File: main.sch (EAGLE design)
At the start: 31 parts, among them IC1 ATTINY13A-SSH, T1A 2N4401, T1B NPN, T2A 2N4401, T2B NPN

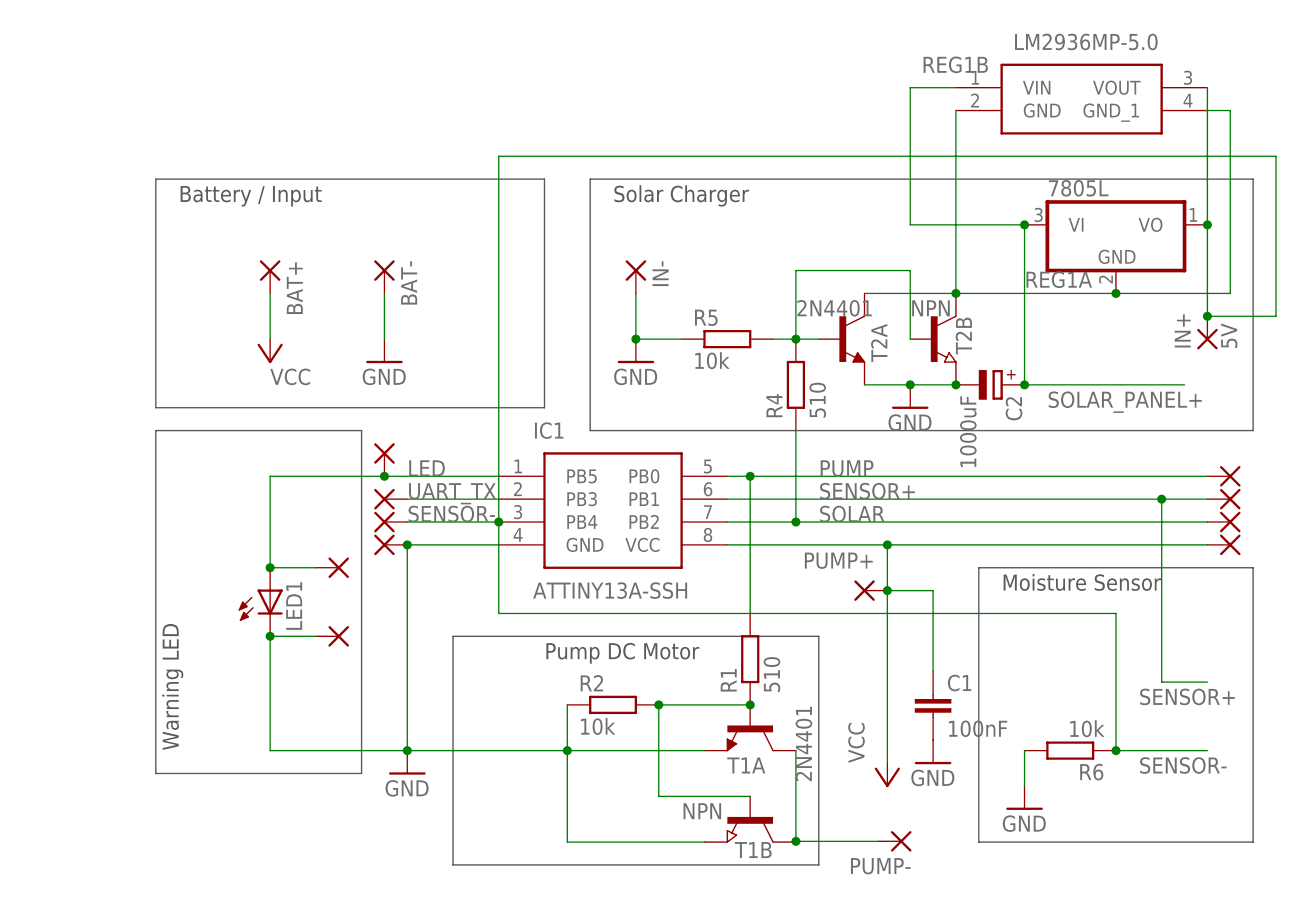
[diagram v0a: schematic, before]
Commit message: rev 0.6
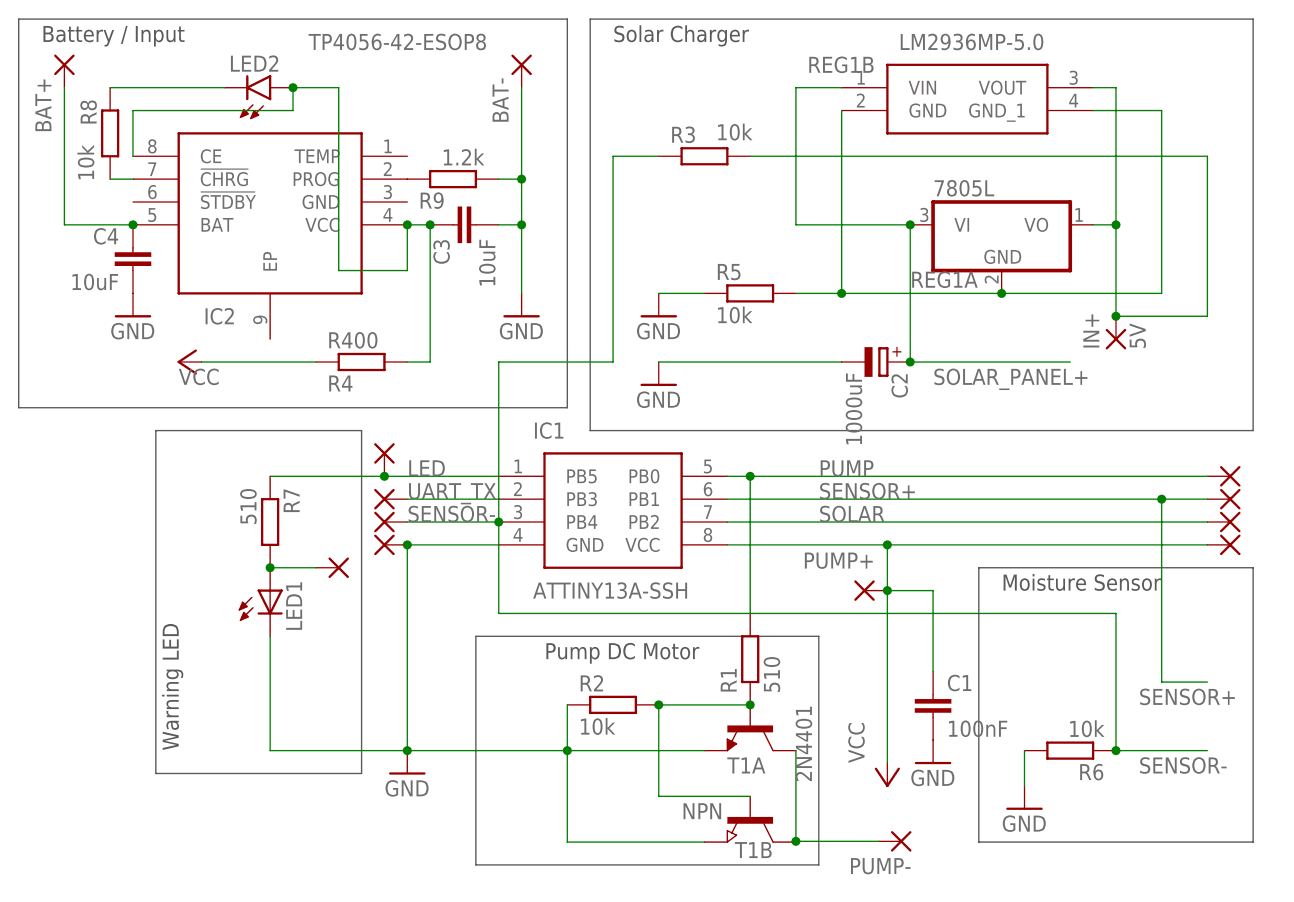
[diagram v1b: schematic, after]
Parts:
- removed IN-: 5V, wirepad:1,6/0,9
- removed PAD2: (no value), wirepad:1,6/0,8
- removed T2A: 2N4401, transistor:-NPN-TO92
- removed T2B: NPN, semicon-smd-ipc:NPN-TRANSISTOR_SOT23W
- added C3, C4: 10uF, rcl:C-EUC3216
- added IC2: TP4056-42-ESOP8, 1EDI60I12AF:TP4056-42-ESOP8
- added LED2: (no value), led:LEDSML0805
- added R3: 10k, resistor:R-EU_M0805
- added R7: 510, resistor:R-EU_M0805
- added R8: 10k, rcl:R-EU_R0603
- added R9: 1.2k, rcl:R-EU_R0603
- R4: value 510 -> R400; device resistor:R-EU_M0805 -> resistor:R-EU_M1206
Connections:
- new net N$11: IC2.PROG, R9.1
- new net N$3: IN+.P, R3.2, REG1A.VO, REG1B.VOUT
- new net N$6: LED1.A, PAD1.P, R7.2
- new net N$7: BAT+.P, C4.1, IC2.BAT
- new net N$8: IC2.!CHRG, R8.2
- new net N$9: LED2.C, R8.1
- net GND: now also C3.2, C4.2, R9.2; no longer IN-.P, PAD2.P, T2A.E, T2B.E
- net LED: now also R7.1; no longer LED1.A, PAD1.P
- net N$4: now also C3.1, IC2.CE, IC2.VCC, LED2.A; no longer R5.2, T2A.B, T2B.B
- net N$5: now also R5.2; no longer T2A.C, T2B.C
- net SENSOR-: now also R3.1; no longer IN+.P, REG1A.VO, REG1B.VOUT
- net SOLAR: no longer R4.1
- net VCC: now also R4.1; no longer BAT+.P
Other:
- moved on the sheet: BAT+, BAT-, C2, IN+, R4, R5, REG1A, REG1B
